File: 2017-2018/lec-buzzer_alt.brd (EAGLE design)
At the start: 60 x 29.5 mm, 27 parts, among them K1 SKQGADE010, K2 SKQGADE010, K3 SKQGADE010, U1 ATMEGA328P-MUR, X1 MINI-USB-32005-201

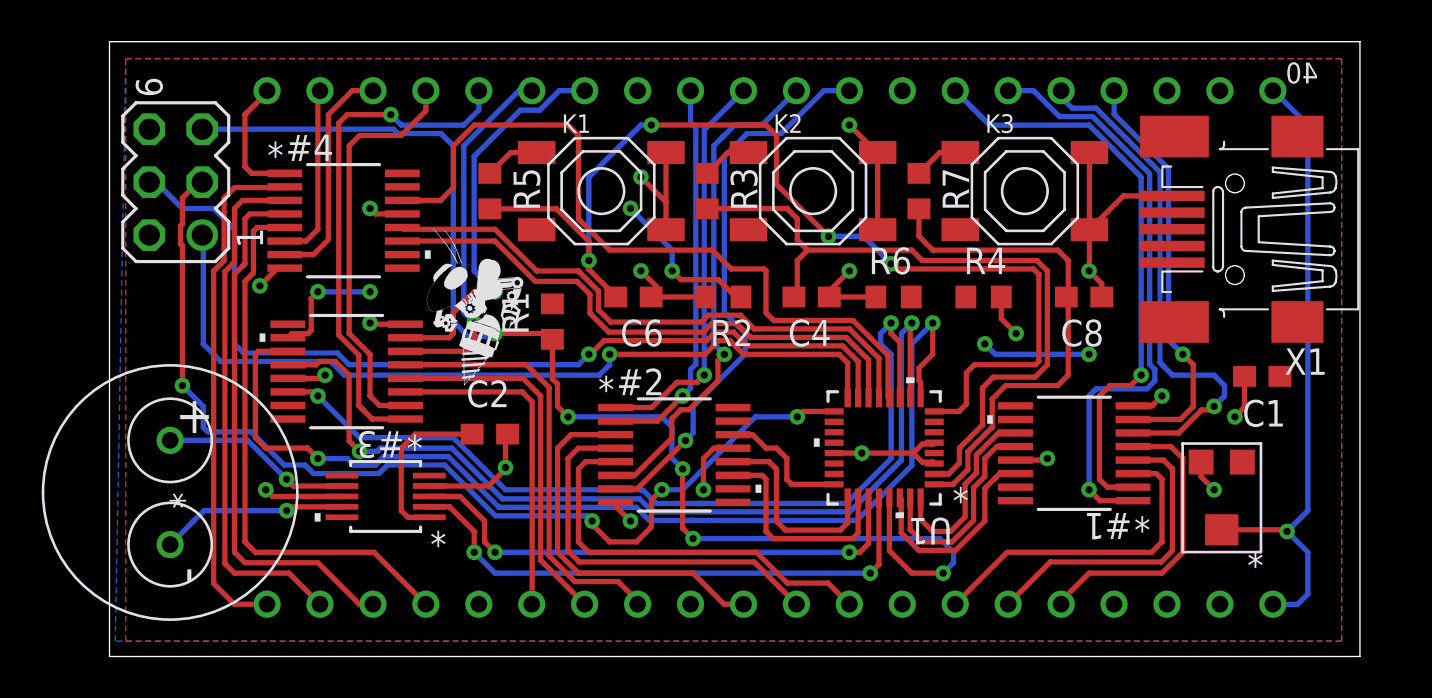
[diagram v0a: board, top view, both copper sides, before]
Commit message: Board Updated according to Design Review
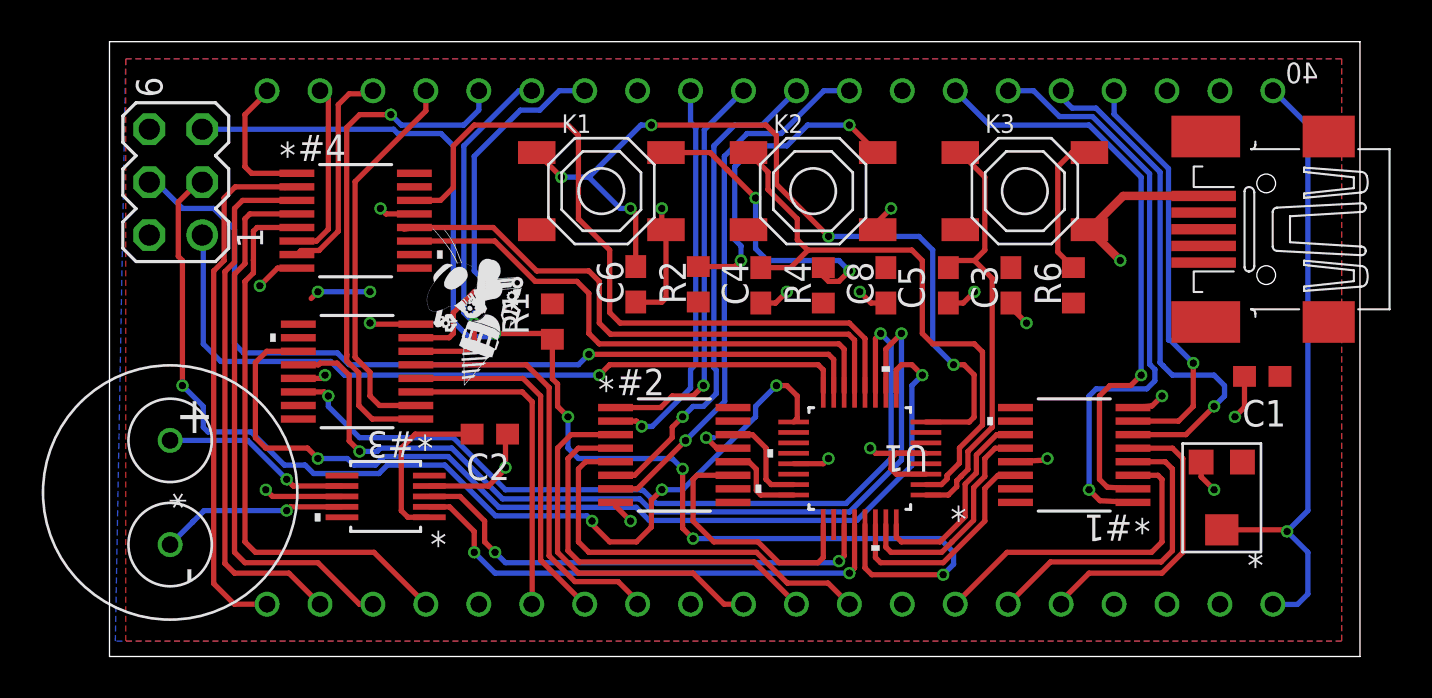
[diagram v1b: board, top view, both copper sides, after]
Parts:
- removed R3, R5, R7: 7.8k, resistor:R0603
- added C3, C5: 0.1uF, rcl:C0603
- C1: value 47uF -> 10uF
- U1: value ATMEGA328P-MUR -> ATMEGA328P-AUR; device lcd-buzzer:32M1-A -> lcd-buzzer:32A
- moved R6 8.65 mm to (58.2, 32.3), turned to 270 degrees
- moved R4 7.71 mm to (46.2, 32.3), turned to 270 degrees
- moved C8 6.53 mm to (52.2, 32.3), turned to 270 degrees
- moved C4 2.50 mm to (43.2, 32.3), turned to 270 degrees
- moved X1 1.50 mm to (67.5, 35.0)
- moved R2 1.35 mm to (40.2, 32.4), turned to 270 degrees
- moved U1 1.28 mm to (48.0, 24.0)
- moved C6 0.62 mm to (37.2, 32.4), turned to 270 degrees
- moved #4 0.58 mm to (23.8, 35.4)
- moved #3 0.50 mm to (23.9, 28.2)
- moved #1 0.08 mm to (58.3, 24.2)
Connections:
- removed net N$1: K2.1, R3.1
- removed net N$2: K1.1, R5.1
- removed net N$4: K3.1, R7.1
- new net N$5: K2.2, R2.1
- new net N$6: K1.2, R4.1
- new net N$7: K3.2, R6.1
- net !BTN1: now also K1.1; no longer R5.2
- net !BTN2: now also K2.1; no longer R3.2
- net !BTN3: now also K3.1; no longer R7.2
- net +5V: now also C3.1, C5.1
- net GND: now also C3.2, C5.2; no longer K1.2, K2.2, K3.2, R2.1, R4.1, R6.1
- net SFT2: now also U1.23; no longer U1.24
- net SHIFT_CLK2: now also U1.24; no longer U1.25
- net STORAGE_CLK2: now also U1.25; no longer U1.26
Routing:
- net +5V: track 18.6 -> 2.96 mm, vias 6 -> 2
- net N$5: track 0.00 -> 15.0 mm, vias 0 -> 2
- net N$6: track 0.00 -> 14.6 mm, vias 0 -> 2
- net GND: track 66.9 -> 56.7 mm, vias 19 -> 21
- net !BTN1: track 50.6 -> 41.4 mm, vias 4 -> 5
- net N$7: track 0.00 -> 6.95 mm
- net !BTN2: track 34.7 -> 28.9 mm
- net SHIFT_CLK2: track 9.66 -> 4.17 mm
- net STORAGE_CLK3: track 51.5 -> 47.6 mm
- net !BTN3: track 24.4 -> 20.8 mm
- net MISO: track 39.9 -> 37.0 mm
- net N$2: track 2.66 -> 0.00 mm
- net N$4: track 2.39 -> 0.00 mm
- net N$1: track 2.39 -> 0.00 mm
- net SCL: track 26.8 -> 24.5 mm
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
